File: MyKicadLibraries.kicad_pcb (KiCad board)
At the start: 2 copper layers, 308 x 139.2 mm, 39 parts, among them J1 Conn_01x08, J10 RCJ-22, J11 DIN-5, J12 Mini-DIN-6, J13 USB_A, J14 Conn_01x02, J15 Conn_01x02, J2 Conn_01x08, J3 POGO Pins, J4 c8-inlet, J5 FTDI, J6 Micro_SD_Card, J7 Conn_01x04, J8 Conn_02x04_Counter_Clockwise, J9 Conn_01x04, SW1 Schurter Switch, U1 radio-receiver, U10 rdm-6300, U11 magnetic-charger, U12 adafruit-MAX98357, U13 TTL, U14 lxb18, U15 esp32-wemos-d1-mini, U16 TCRT5000, U17 opb607a, U18 max98367, U19 esp-01f, U2 tp4056, U20 m18, U21 bme280, U3 LilygoSIMT7000G, U4 esp-01m, U5 relais_module, U6 ESP-01, U7 dcdc, U8 mems-mic, U9 ESP-12E

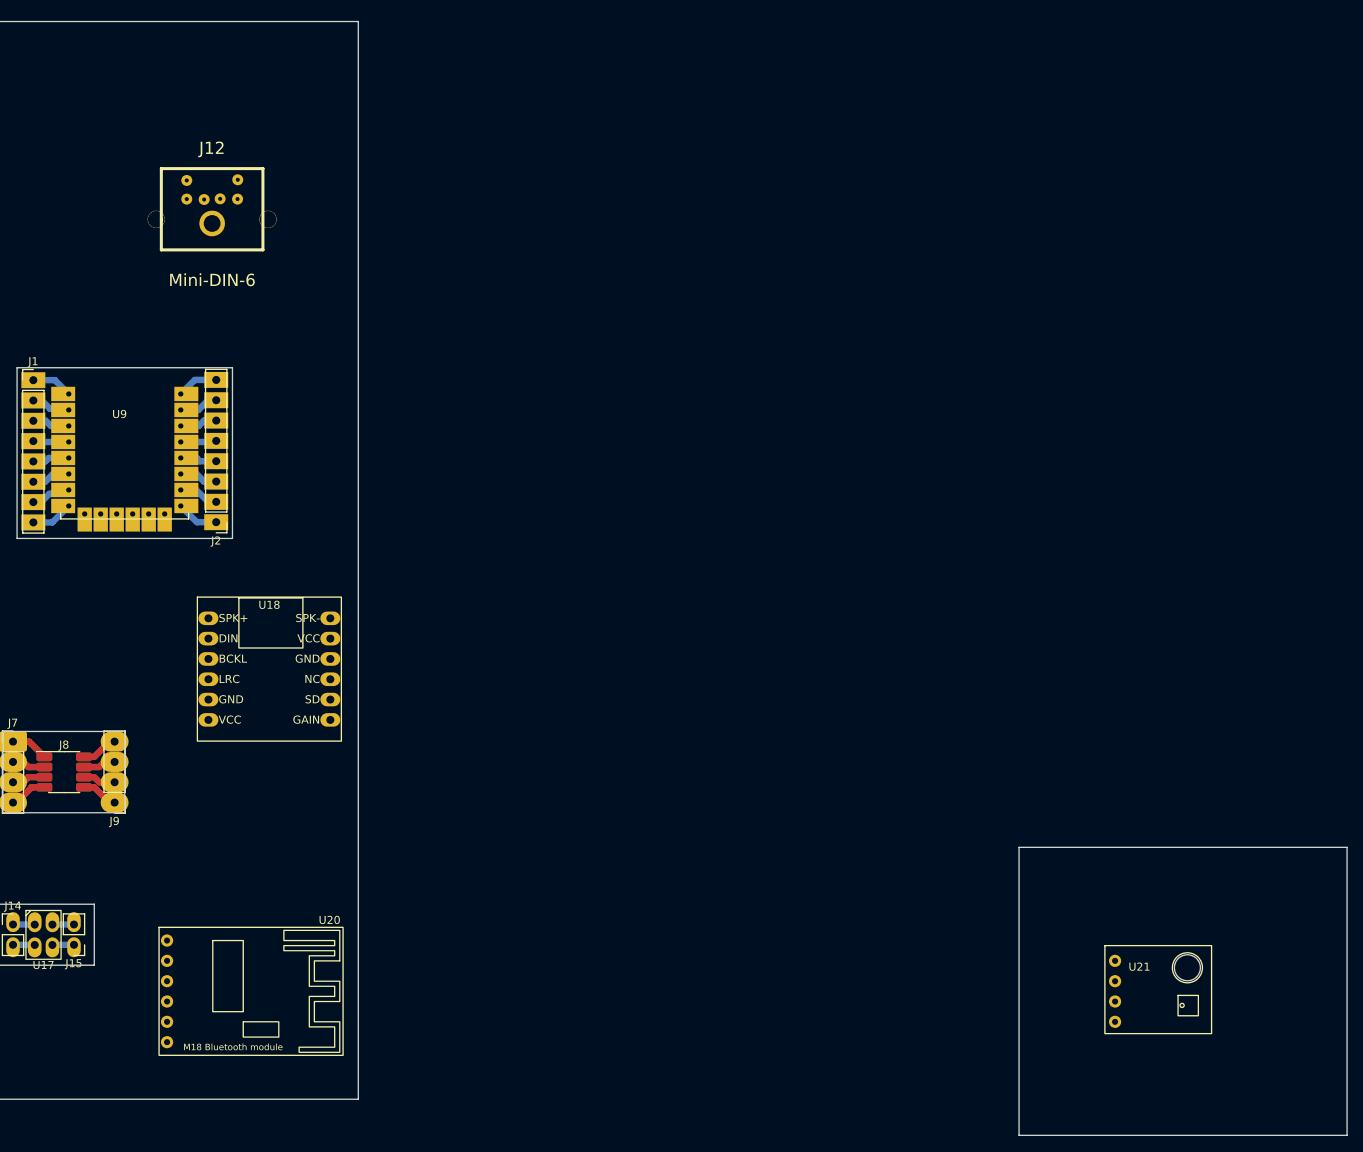
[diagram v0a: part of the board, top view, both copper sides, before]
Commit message: Update main file
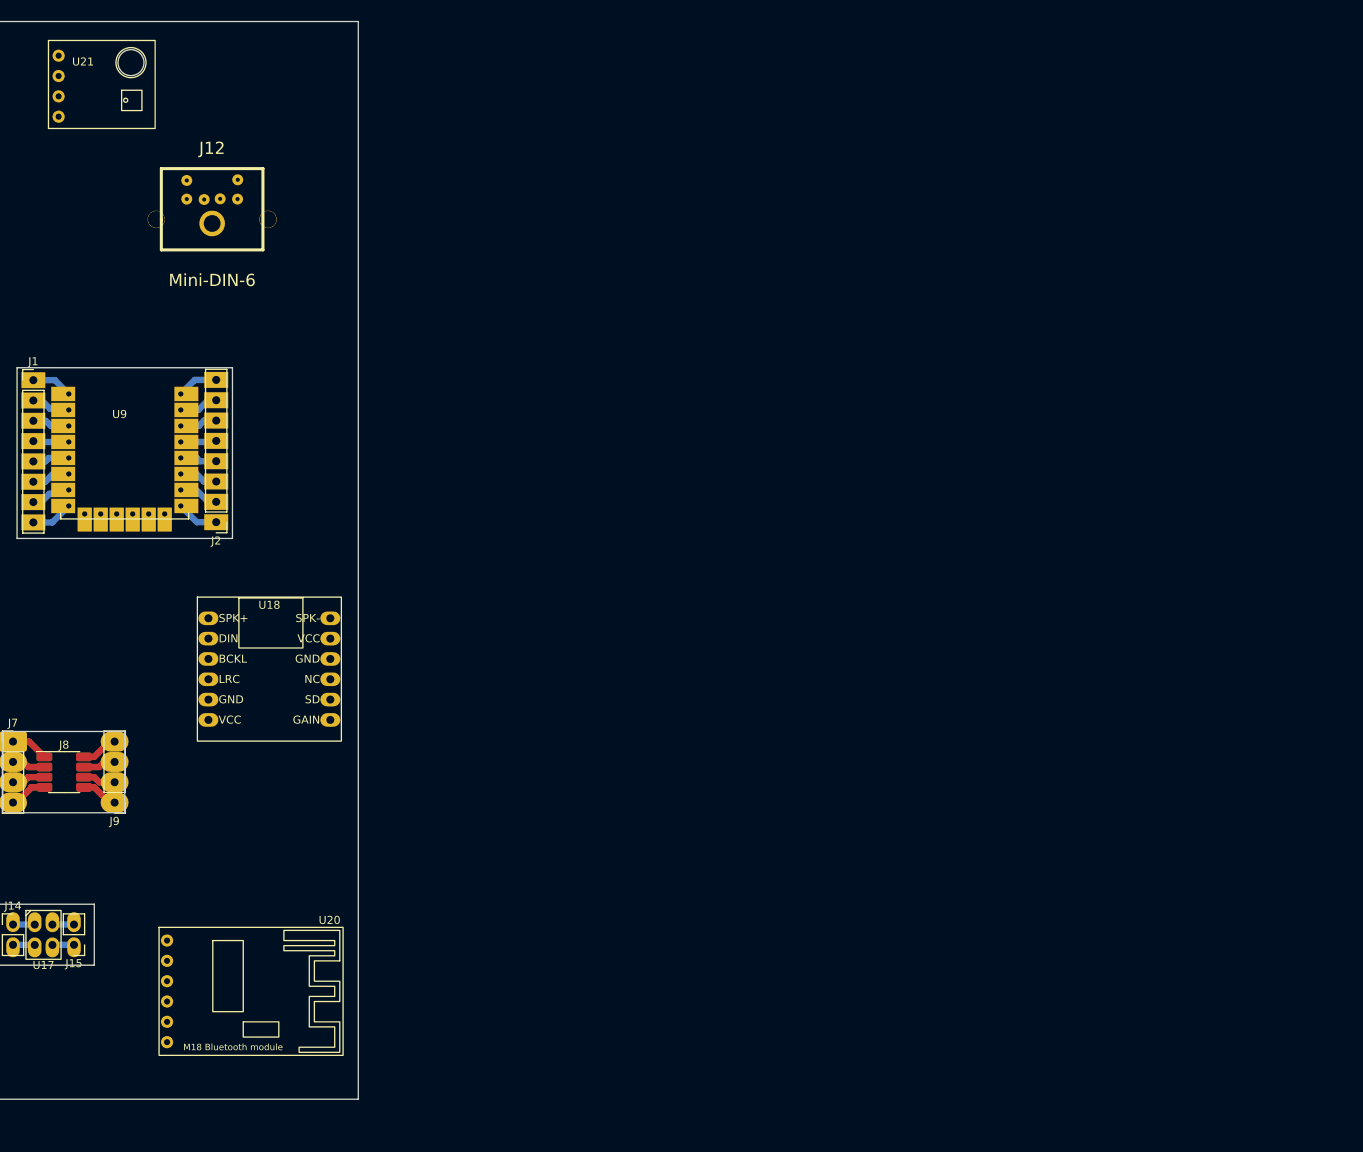
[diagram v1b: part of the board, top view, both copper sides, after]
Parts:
- moved U21 173.9 mm to (214.9, 40.9)
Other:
- board size 308 x 139.2 mm -> 184.4 x 134.7 mm
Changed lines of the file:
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@@
   )
   (footprint "bme280:bme280" (layer "F.Cu")
-    (at 347 154)
+    (at 214.9475 40.855)
     (property "Sheetfile" "MyKicadLibraries.kicad_sch")
     (property "Sheetname" "")
@@
   (gr_rect (start 206.705 143.105) (end 219.405 150.725) (layer "Edge.Cuts") (width 0.1) (fill none))
   (gr_rect (start 68.042948 32.770045) (end 252.405 167.485) (layer "Edge.Cuts") (width 0.1) (fill none))
-  (gr_rect (start 335 136) (end 376 172) (layer "Edge.Cuts") (width 0.1) (fill none))
   (segment (start 72.593 104.497) (end 90.881 104.497) (width 0.8) (layer "F.Cu") (net 82))
   (segment (start 72.593 97.385) (end 90.881 97.385) (width 0.8) (layer "F.Cu") (net 83))
